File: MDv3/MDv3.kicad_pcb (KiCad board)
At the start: 2 copper layers, 42 parts, among them J1 XT60PW-M, J2 XT60PW-M, J3 XT30PW-M, J4 XT30PW-M

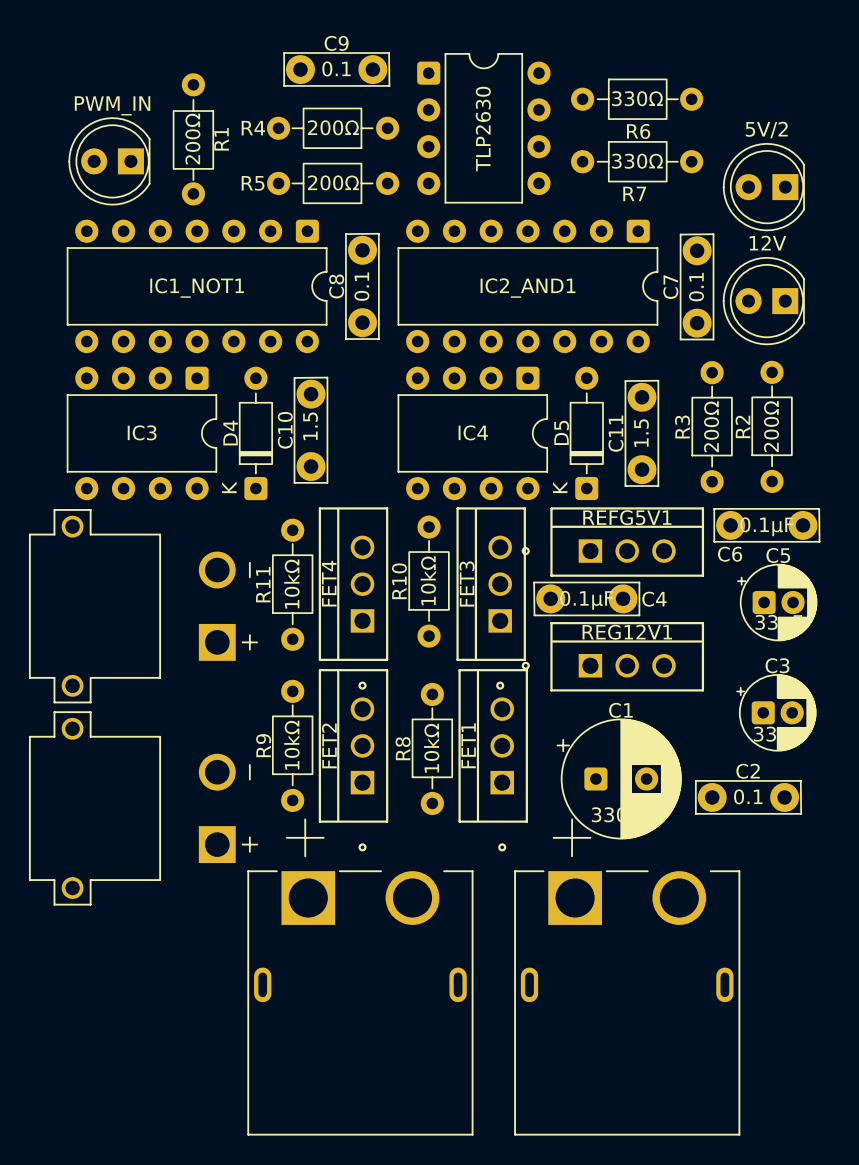
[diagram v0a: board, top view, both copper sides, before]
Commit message: 本当の配線前
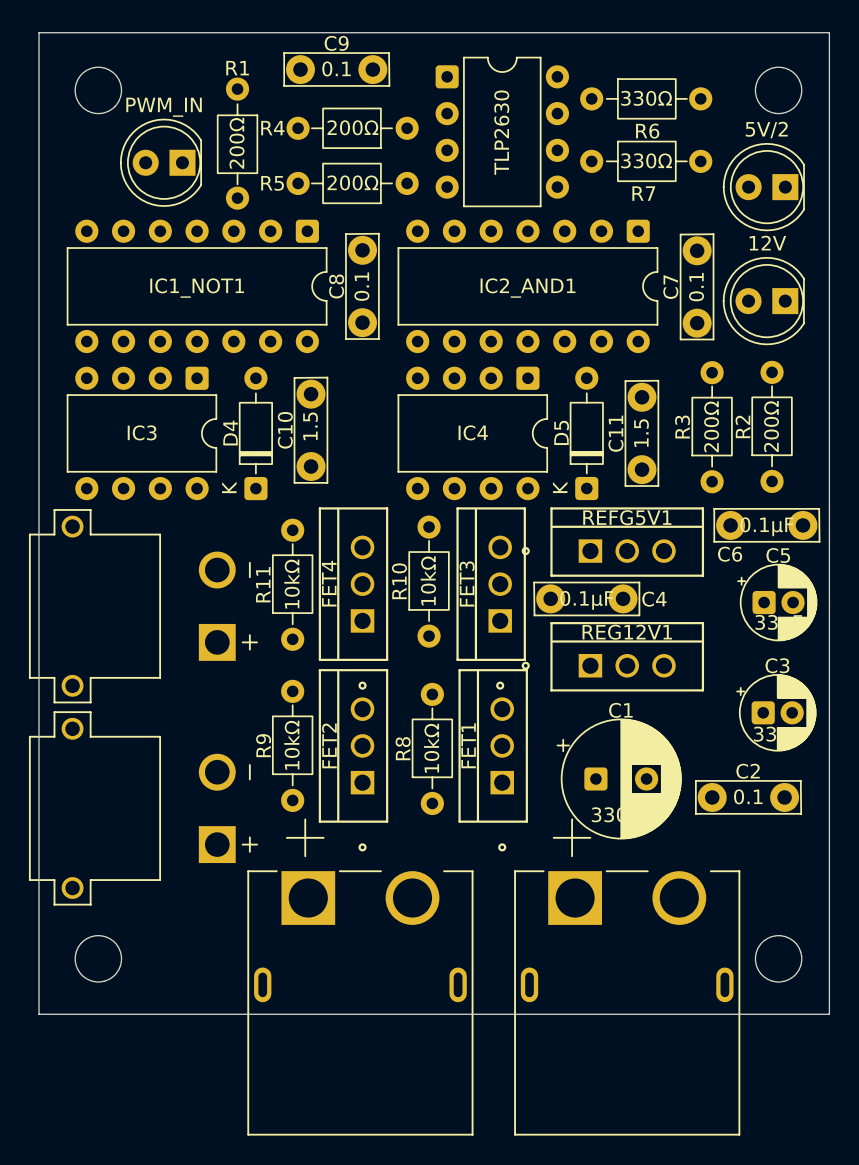
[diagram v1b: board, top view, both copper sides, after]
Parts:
- added REF**: MountingHole_3.2mm_M3, MountingHole:MountingHole_3.2mm_M3, F.Cu at (140.0, 116.0)
- added REF**: MountingHole_3.2mm_M3, MountingHole:MountingHole_3.2mm_M3, F.Cu at (93.0, 116.0)
- added REF**: MountingHole_3.2mm_M3, MountingHole:MountingHole_3.2mm_M3, F.Cu at (93.0, 176.0)
- added REF**: MountingHole_3.2mm_M3, MountingHole:MountingHole_3.2mm_M3, F.Cu at (140.0, 176.0)
- moved D1 3.56 mm to (98.8, 121.0)
- moved R1 3.06 mm to (102.6, 115.9)
- moved R4 1.35 mm to (114.3, 118.6)
- moved R5 1.35 mm to (114.3, 122.5)
- moved TLP2630 1.30 mm to (117.1, 115.1)
- moved R6 0.63 mm to (127.1, 116.6)
- moved R7 0.63 mm to (127.1, 120.9)
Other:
- board outline added: 54.6 x 67.8 mm
